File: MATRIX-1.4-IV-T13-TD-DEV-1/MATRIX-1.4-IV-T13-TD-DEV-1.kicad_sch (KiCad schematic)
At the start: 153 parts, among them Q401 MPSA42, Q402 MPSA42, Q403 MPSA92, Q404 MPSA92, Q405 MJE340, Q406 MJE350, Q407 MJE350, Q408 MJE340, Q409 MJE15032, Q410 MJE15033, Q411 2SC5200, Q412 2SA1943, Q4131 2SC5200, Q4132 2SC5200, Q4133 2SC5200, Q4134 2SC5200, Q4135 2SC5200, Q4136 2SC5200, Q4141 2SA1943, Q4142 2SA1943, Q4143 2SA1943, Q4144 2SA1943, Q4145 2SA1943, Q4146 2SA1943, Q601 2N5401, Q602 MJE340, Q603 MJE15032, Q604 2SC5200, Q605 2N5401, Q606 MJE340, Q607 2N5401, Q608 2N5401, Q701 2N5551, Q702 MJE350, Q703 MJE15033, Q704 2SA1943, Q705 2N5551, Q706 MJE350, Q707 2N5551, Q708 2N5551

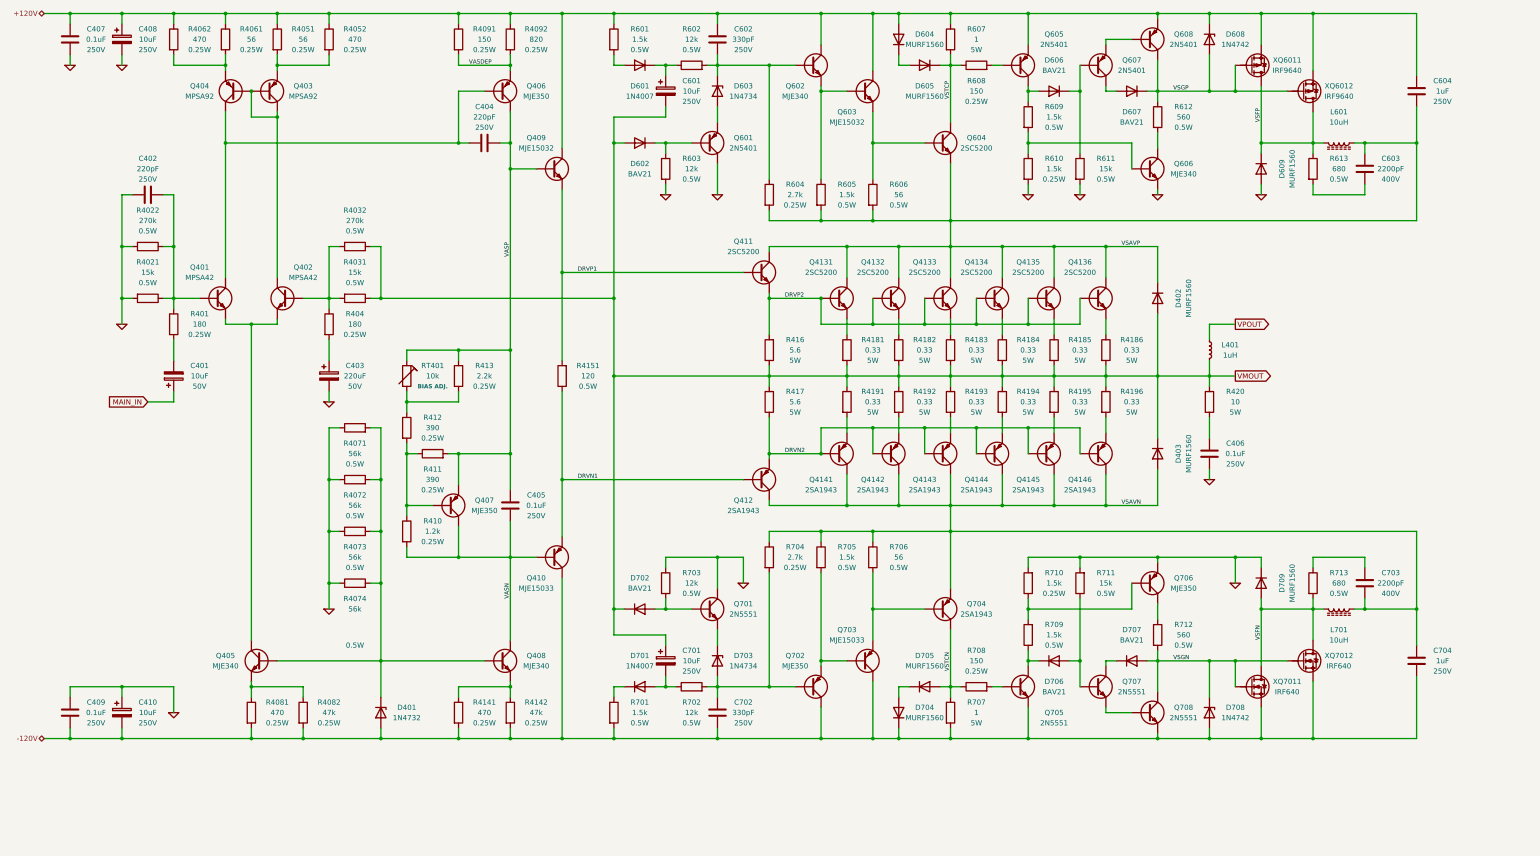
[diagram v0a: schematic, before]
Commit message: Routine Update Sat Jul 23 04:17:04 PM WIB 2022
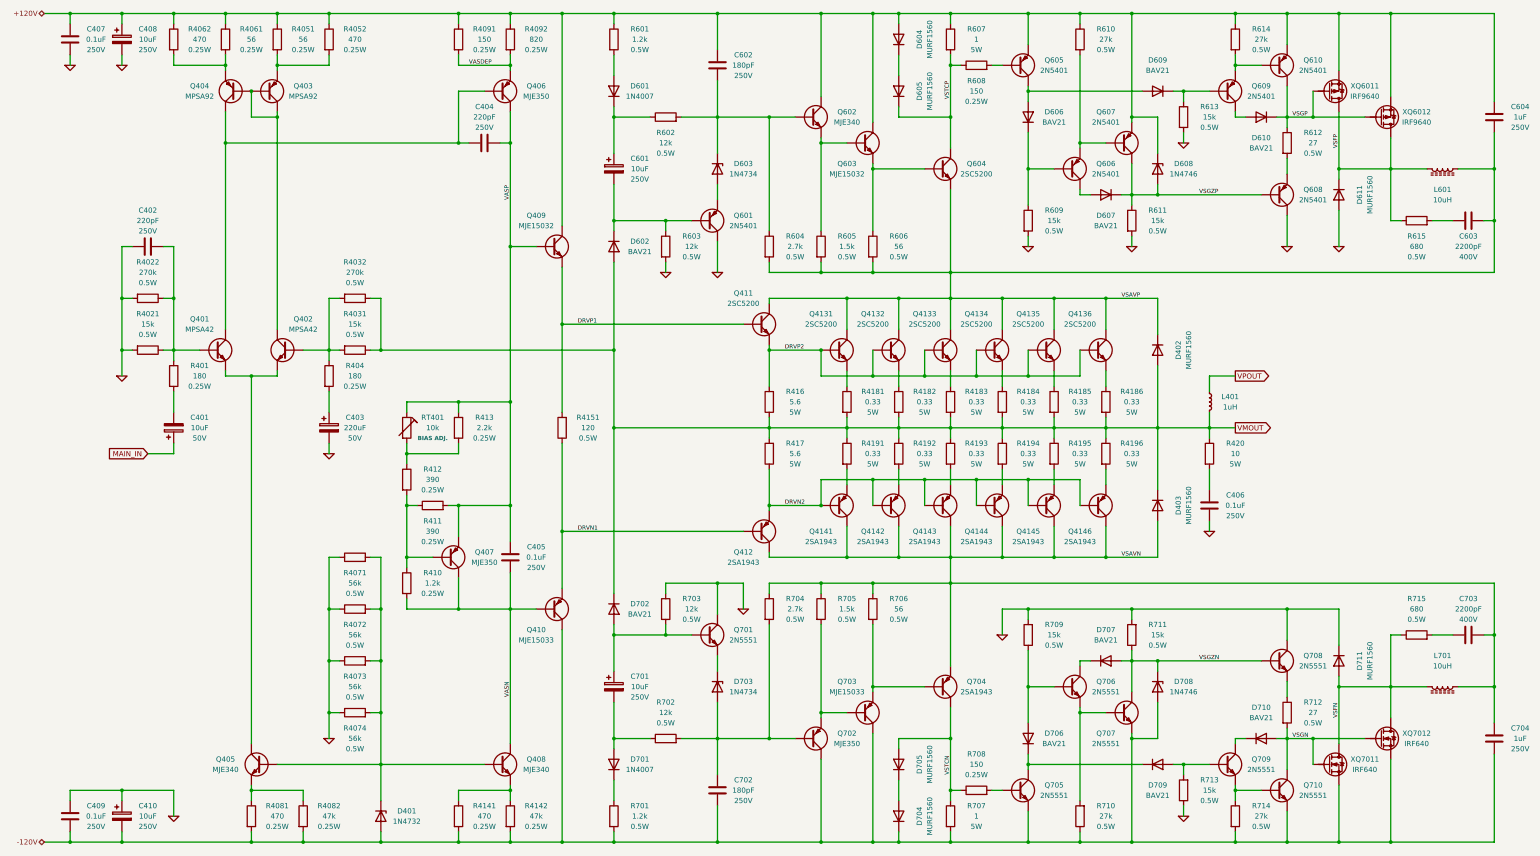
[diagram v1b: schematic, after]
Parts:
- removed Q606: MJE340, MATRIX_1.4:TO-225, symbol MATRIX_1.4:Q_NPN_CBE
- removed Q706: MJE350, MATRIX_1.4:TO-225, symbol MATRIX_1.4:Q_PNP_CBE
- removed R609: 1.5k, MATRIX_1.4:RESISTOR_AXIAL_0.5W, symbol Device:R
- removed R713: 680, MATRIX_1.4:RESISTOR_AXIAL_0.5W, symbol Device:R
- added D606, D607, D706, D707: BAV21, MATRIX_1.4:DIODE_AXIAL_SMALL_GE, symbol MATRIX_1.4:D
- added Q606, Q607, Q608: 2N5401, MATRIX_1.4:TO-92-EBC, symbol MATRIX_1.4:Q_PNP_CBE
- added Q706, Q707, Q708: 2N5551, MATRIX_1.4:TO-92-EBC, symbol MATRIX_1.4:Q_NPN_CBE
- added R610, R614, R714: 27k, MATRIX_1.4:RESISTOR_AXIAL_0.5W, symbol Device:R
- added R611, R711: 15k, MATRIX_1.4:RESISTOR_AXIAL_0.5W, symbol Device:R
- added R715: 680, MATRIX_1.4:RESISTOR_AXIAL_0.5W, symbol Device:R
- C602, C702: value 330pF -> 180pF
- D608, D708: value 1N4742 -> 1N4746; Spice_Model 1N4742 -> 1N4746
- R601, R701: value 1.5k -> 1.2k
- R604, R704: footprint MATRIX_1.4:RESISTOR_AXIAL_0.25W -> MATRIX_1.4:RESISTOR_AXIAL_0.5W; Wattage 0.25W -> 0.5W
- R609: renamed from R610; value 1.5k -> 15k; footprint MATRIX_1.4:RESISTOR_AXIAL_0.25W -> MATRIX_1.4:RESISTOR_AXIAL_0.5W; Wattage 0.25W -> 0.5W
- R612, R712: value 560 -> 27
- R709: value 1.5k -> 15k
- R710: value 1.5k -> 27k; footprint MATRIX_1.4:RESISTOR_AXIAL_0.25W -> MATRIX_1.4:RESISTOR_AXIAL_0.5W; Wattage 0.25W -> 0.5W
- renumbered D606 to D609, D607 to D610, D609 to D611, D706 to D709, D707 to D710, D709 to D711, Q607 to Q609, Q608 to Q610, Q707 to Q709, Q708 to Q710, R611 to R613, R613 to R615, R711 to R713
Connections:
- net +120V: now also Q607.3 (E), R610.1, R614.1
- net -120V: now also R710.1, Q707.3 (E), R714.2
- net 0: now also R709.2, R713.1, Q608.1 (C), Q708.1 (C), R611.2, R711.2; no longer R710.2, R713.2
- net VMOUT: no longer C601.2, C701.1
- net VSAVP: now also C603.1; no longer C603.2
- net VSFN: now also R715.1
- net VSGN: no longer D708.2 (K)
- net VSGP: no longer D608.1 (A)
- net at D709.1 (A), Q709.2 (B): now also R713.2; no longer R713.1
- net at Q709.3 (E), Q710.2 (B): now also R714.1
- net at R712.1: now also Q708.3 (E)
- net at D709.2 (K), Q705.1 (C): now also D706.2 (K); no longer R709.1
- net at R612.2: now also Q608.3 (E)
- net at D602.2 (K), Q601.2 (B), R603.1: now also C601.2
- net at D702.1 (A), Q701.2 (B), R703.2: now also C701.1
- net at D609.1 (A), Q605.1 (C): now also D606.1 (A)
- net at C703.2: now also R715.2
- net at R609.1: now also D606.2 (K), Q606.2 (B)
- net at Q609.3 (E), Q610.2 (B): now also R614.2
- net at R615.2: now also C603.2; no longer C603.1
- new net: D707.2 (K), Q706.1 (C)
- new net: D706.1 (A), Q706.2 (B), R709.1
- new net: Q706.3 (E), Q707.2 (B), R710.2
- new net: D607.1 (A), Q606.1 (C)
- new net: Q606.3 (E), Q607.2 (B), R610.2
- new net VSGZN: D707.1 (A), D708.2 (K), Q707.1 (C), Q708.2 (B), R711.1
- new net VSGZP: D607.2 (K), D608.1 (A), Q607.1 (C), Q608.2 (B), R611.1
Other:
- moved on the sheet: C401, C402, C403, C405, C406, C409, C410, C601, C602, C603, C604, C701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
